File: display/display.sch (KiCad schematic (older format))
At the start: 37 parts, among them J1 Conn_01x02, J2 Conn_01x03, J3 Conn_01x05

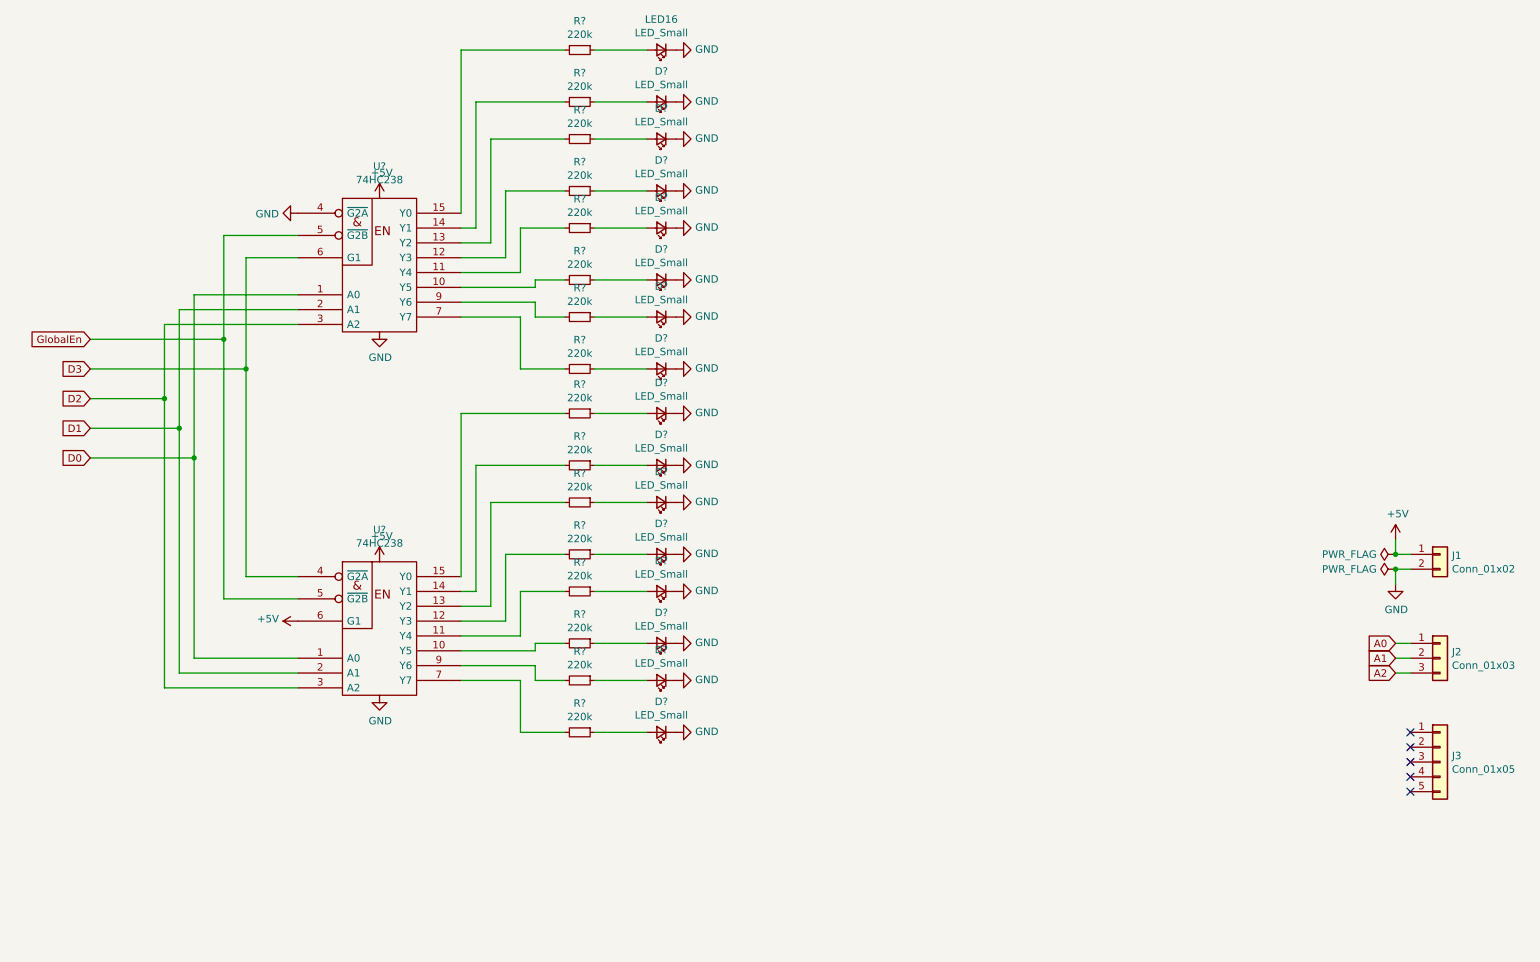
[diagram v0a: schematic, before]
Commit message: display board template
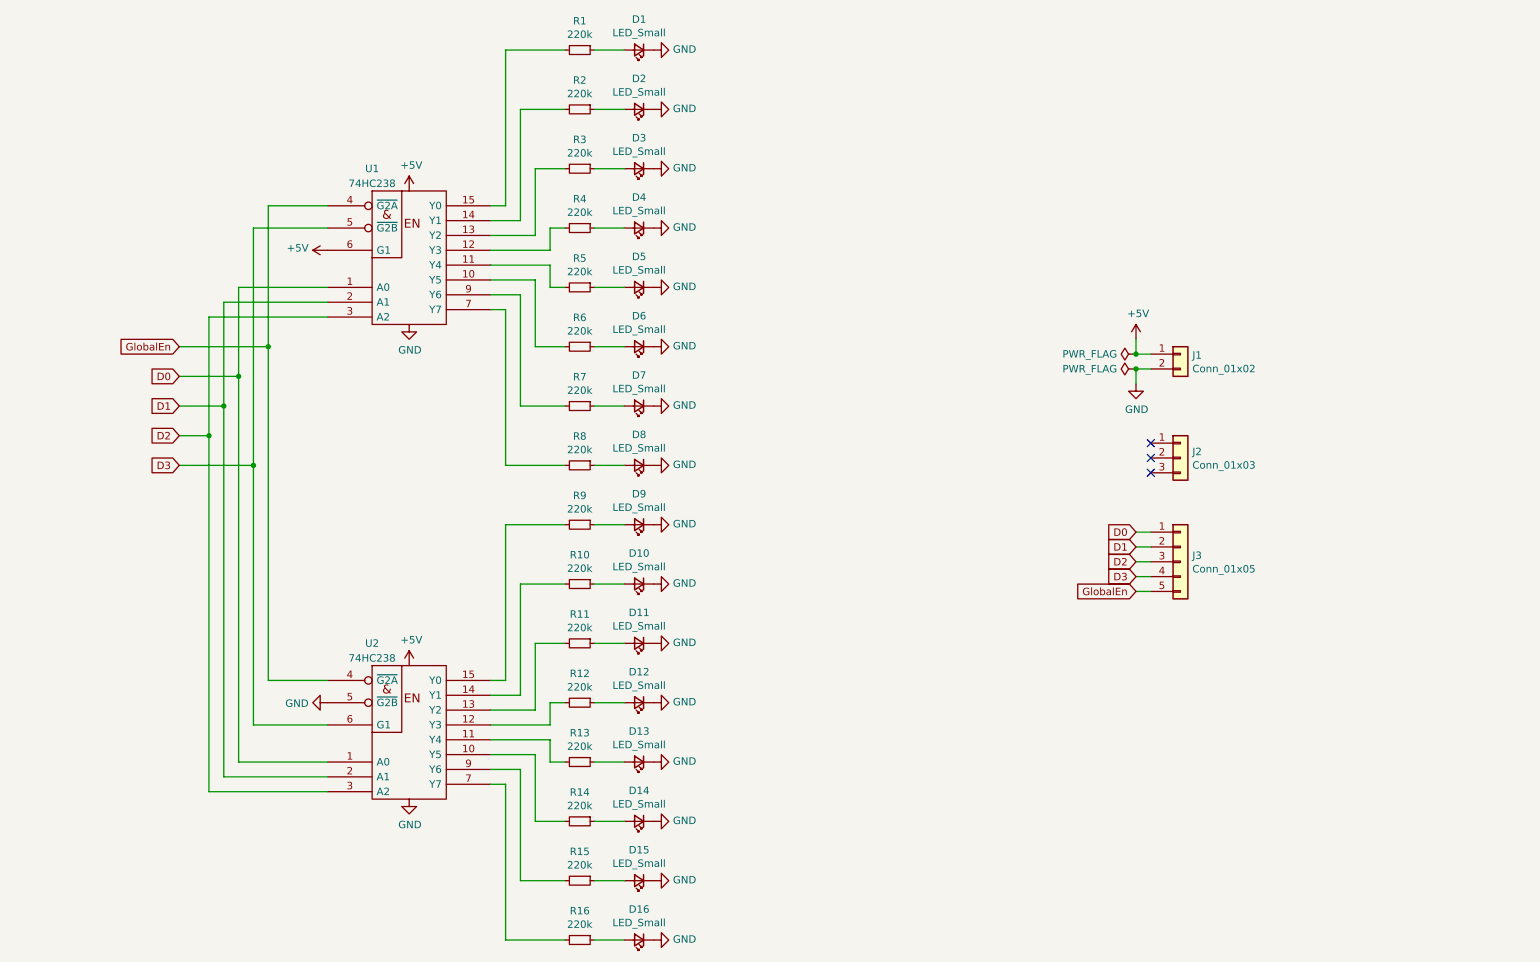
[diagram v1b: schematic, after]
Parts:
- removed D? (x14): LED_Small, symbol Device:LED_Small
- removed R? (x14): 220k, symbol Device:R_Small
- removed U?: 74HC238, symbol 74xx_IEEE:74HC238
- added D10, D11, D12, D13, D14, D15, D16, D3, D4, D5, D6, D7, D8, D9: LED_Small, LED_THT:LED_D5.0mm, symbol Device:LED_Small
- added R10, R11, R12, R13, R14, R15, R16, R3, R4, R5, R6, R7, R8, R9: 220k, Resistor_SMD:R_0603_1608Metric, symbol Device:R_Small
- added U2: 74HC238, Package_SO:SOIC-16_3.9x9.9mm_P1.27mm, symbol 74xx_IEEE:74HC238
- D1: renamed from LED16; footprint (none) -> LED_THT:LED_D5.0mm
- D2: renamed from D?; footprint (none) -> LED_THT:LED_D5.0mm
- R1, R2: renamed from R?; footprint (none) -> Resistor_SMD:R_0603_1608Metric
- U1: renamed from U?; footprint (none) -> Package_SO:SOIC-16_3.9x9.9mm_P1.27mm
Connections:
- net +5V: now also U1.6 (G1), U2.16 (VCC)
- net D0: now also J3.1 (Pin_1), U2.1 (A0)
- net D1: now also J3.2 (Pin_2), U2.2 (A1)
- net D2: now also J3.3 (Pin_3), U2.3 (A2)
- net D3: now also J3.4 (Pin_4), U1.5 (~G2B), U2.6 (G1); no longer U1.6 (G1)
- net GND: now also D10.1 (K), D11.1 (K), D12.1 (K), D13.1 (K), D14.1 (K), D15.1 (K), D16.1 (K), D3.1 (K), D4.1 (K), D5.1 (K), D6.1 (K), D7.1 (K), D8.1 (K), D9.1 (K), U2.5 (~G2B), U2.8 (GND); no longer U1.4 (~G2A)
- net GlobalEn: now also J3.5 (Pin_5), U1.4 (~G2A), U2.4 (~G2A); no longer U1.5 (~G2B)
- net at U1.10 (Y5): now also R6.2
- net at U1.11 (Y4): now also R5.2
- net at U1.12 (Y3): now also R4.2
- net at U1.13 (Y2): now also R3.2
- net at U1.7 (Y7): now also R8.2
- net at U1.9 (Y6): now also R7.2
- net A0: no longer names the net of J2.1 (Pin_1)
- net A1: no longer names the net of J2.2 (Pin_2)
- net A2: no longer names the net of J2.3 (Pin_3)
- new net: D4.2 (A), R4.1
- new net: D3.2 (A), R3.1
- new net: D6.2 (A), R6.1
- new net: D5.2 (A), R5.1
- new net: D8.2 (A), R8.1
- new net: D7.2 (A), R7.1
- new net: R14.2, U2.10 (Y5)
- new net: R13.2, U2.11 (Y4)
- new net: R12.2, U2.12 (Y3)
- new net: R11.2, U2.13 (Y2)
- new net: R10.2, U2.14 (Y1)
- new net: R9.2, U2.15 (Y0)
- new net: R16.2, U2.7 (Y7)
- new net: R15.2, U2.9 (Y6)
- new net: D16.2 (A), R16.1
- new net: D15.2 (A), R15.1
- new net: D14.2 (A), R14.1
- new net: D13.2 (A), R13.1
- new net: D12.2 (A), R12.1
- new net: D11.2 (A), R11.1
- new net: D10.2 (A), R10.1
- new net: D9.2 (A), R9.1
- no-connect marks 5 -> 3
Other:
- moved on the sheet: D1, D2, J1, J2, J3, R2, U1

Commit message: errata 2: fix footprints
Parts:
- J1: footprint Connector_PinSocket_2.54mm:PinSocket_1x02_P2.54mm_Vertical -> df-parts:310-XX-102-41-001000
- J2: footprint Connector_PinSocket_2.54mm:PinSocket_1x03_P2.54mm_Vertical -> df-parts:310-XX-103-41-001000
- J3: footprint Connector_PinSocket_2.54mm:PinSocket_1x05_P2.54mm_Vertical -> df-parts:310-XX-105-41-001000
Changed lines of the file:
@@
 F 0 "J1" H 8580 3242 50  0000 L CNN
 F 1 "Conn_01x02" H 8580 3151 50  0000 L CNN
-F 2 "Connector_PinSocket_2.54mm:PinSocket_1x02_P2.54mm_Vertical" H 8500 3250 50  0001 C CNN
+F 2 "df-parts:310-XX-102-41-001000" H 8500 3250 50  0001 C CNN
 F 3 "~" H 8500 3250 50  0001 C CNN
 	1    8500 3250
@@
 F 0 "J2" H 8580 3992 50  0000 L CNN
 F 1 "Conn_01x03" H 8580 3901 50  0000 L CNN
-F 2 "Connector_PinSocket_2.54mm:PinSocket_1x03_P2.54mm_Vertical" H 8500 3950 50  0001 C CNN
+F 2 "df-parts:310-XX-103-41-001000" H 8500 3950 50  0001 C CNN
 F 3 "~" H 8500 3950 50  0001 C CNN
 	1    8500 3950
@@
 F 0 "J3" H 8580 4692 50  0000 L CNN
 F 1 "Conn_01x05" H 8580 4601 50  0000 L CNN
-F 2 "Connector_PinSocket_2.54mm:PinSocket_1x05_P2.54mm_Vertical" H 8500 4650 50  0001 C CNN
+F 2 "df-parts:310-XX-105-41-001000" H 8500 4650 50  0001 C CNN
 F 3 "~" H 8500 4650 50  0001 C CNN
 	1    8500 4650
